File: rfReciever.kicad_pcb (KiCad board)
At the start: 4 copper layers, 22.8 x 36.5 mm, 40 parts, among them J1 MOLEX 1054440001, J2 Conn_01x02, J3 Conn_01x02, J4 Conn_01x03, SW1 RF_RESET, SW2 RF_SLEEP, U1 TLV70130DBVR, U2 USBLC6-2SC6, U3 FT234XD-R, X1 DigiXBeeRX900Micro

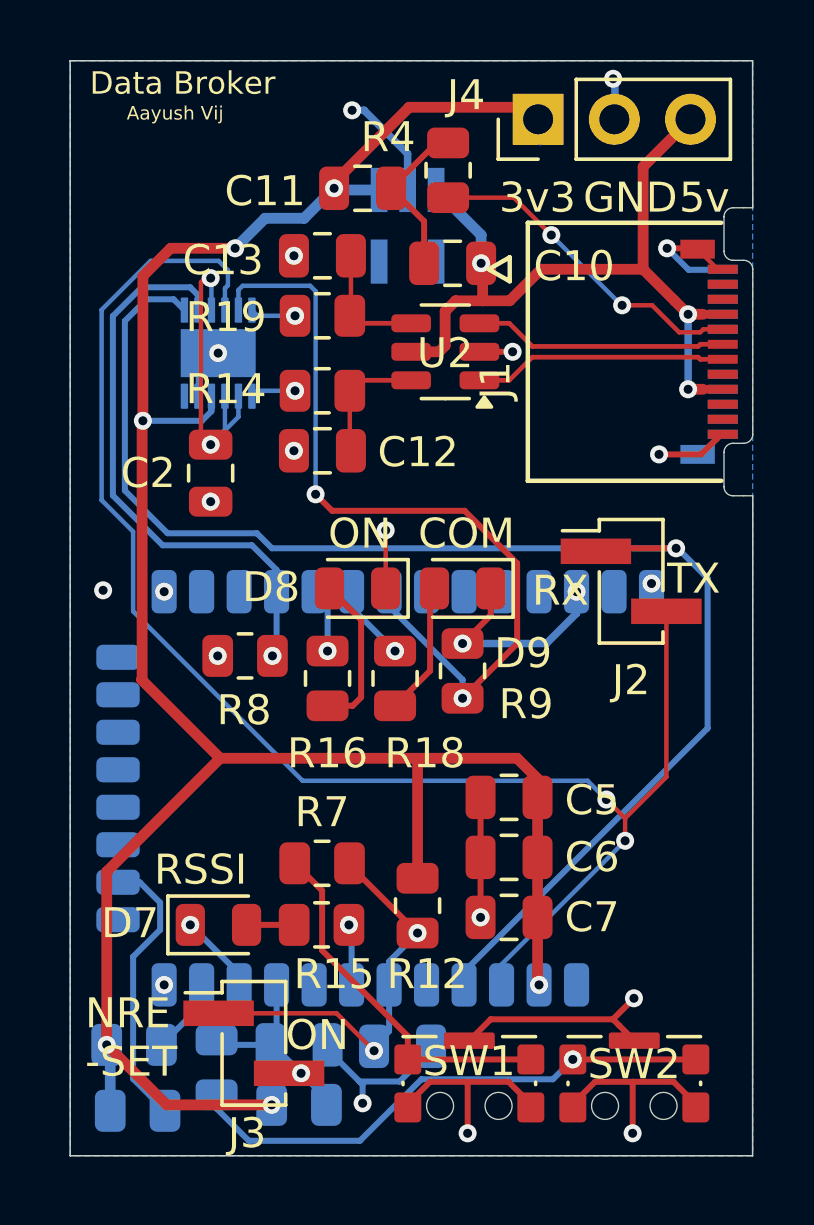
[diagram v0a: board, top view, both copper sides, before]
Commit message: fixed drc
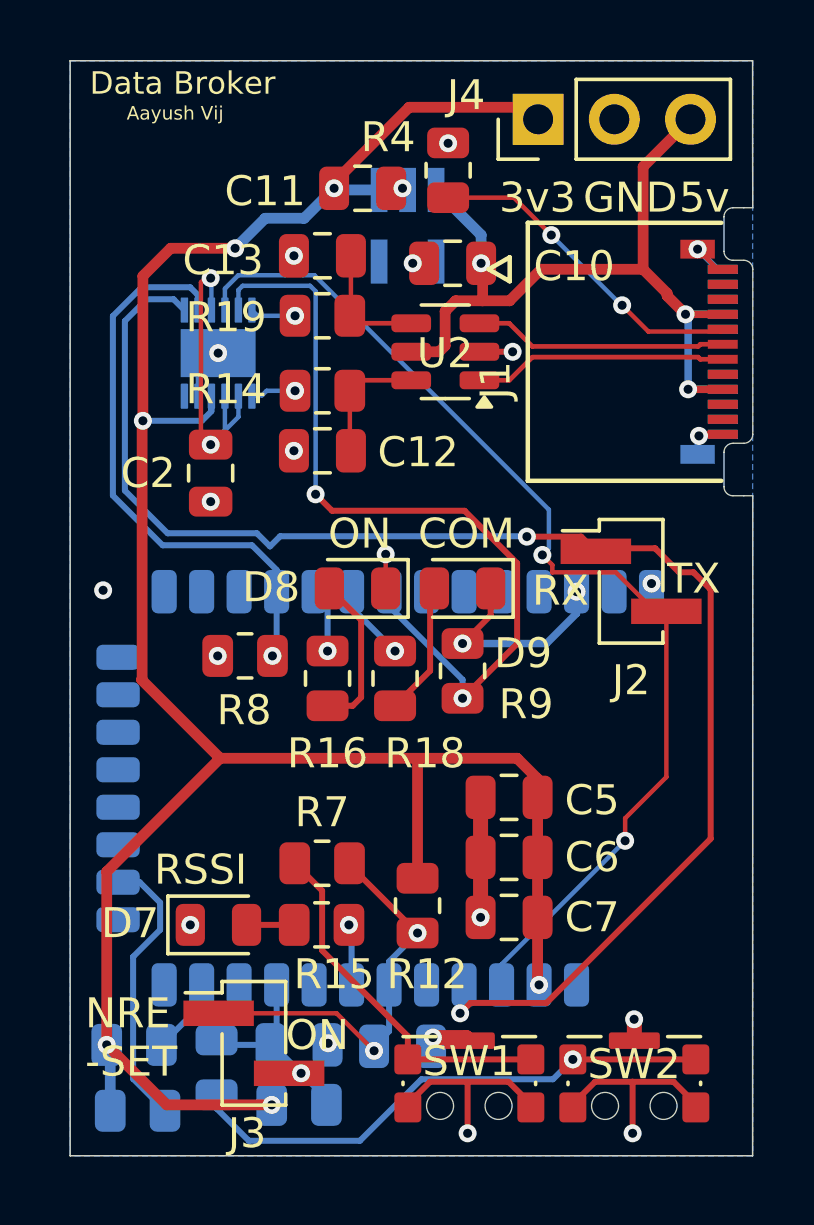
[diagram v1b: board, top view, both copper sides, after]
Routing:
- net GND: track 63.7 -> 35.7 mm
- net /RF_RXD: track 50.9 -> 36.3 mm
- net /RF_TXD: track 48.4 -> 49.4 mm, vias 1 -> 2
- net +5V: track 28.8 -> 29.7 mm
- net +3.3V: track 80.0 -> 79.2 mm
